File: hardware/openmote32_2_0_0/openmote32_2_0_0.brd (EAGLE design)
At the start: 24.1 x 32.8 mm, 39 parts, among them J1 XBEE_1-10, J2 XBEE_11-20, J3 JTAG_CONNECTOR, U1 AT86RF231, X1 16MHz

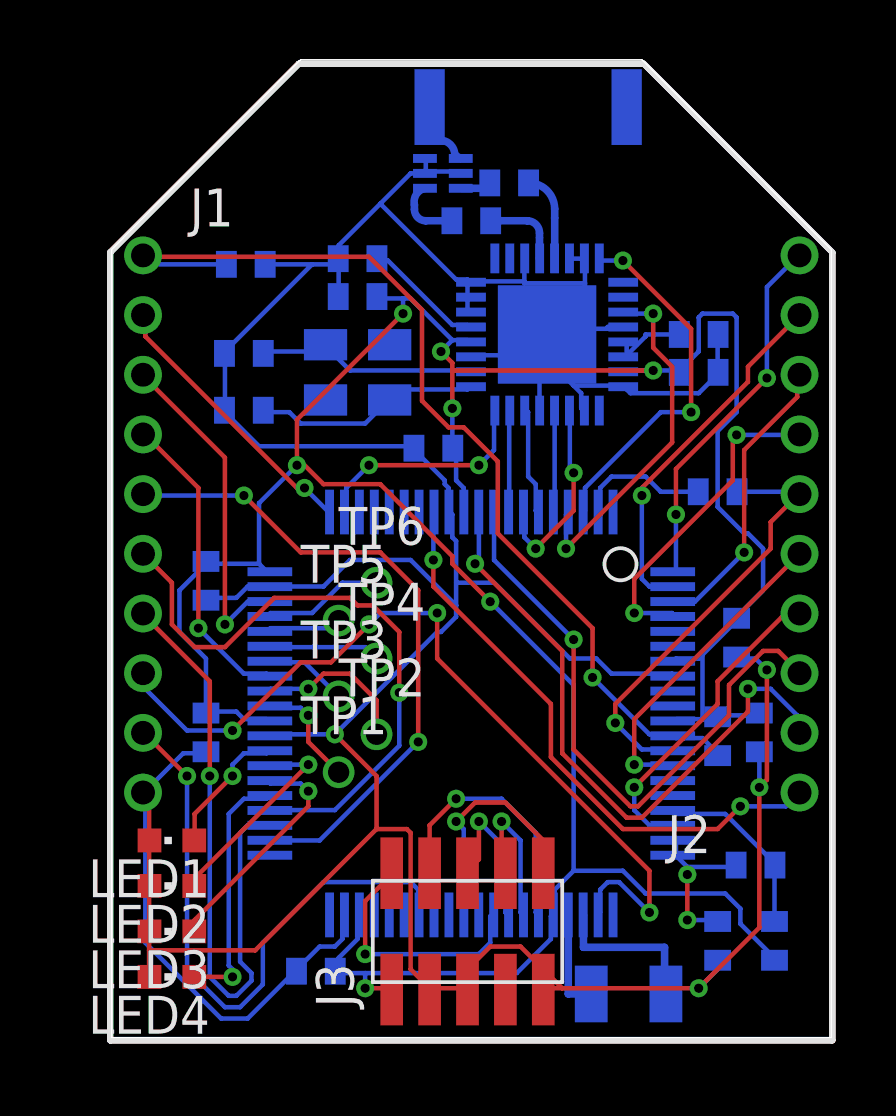
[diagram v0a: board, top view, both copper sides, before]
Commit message: Openmote v2 changes
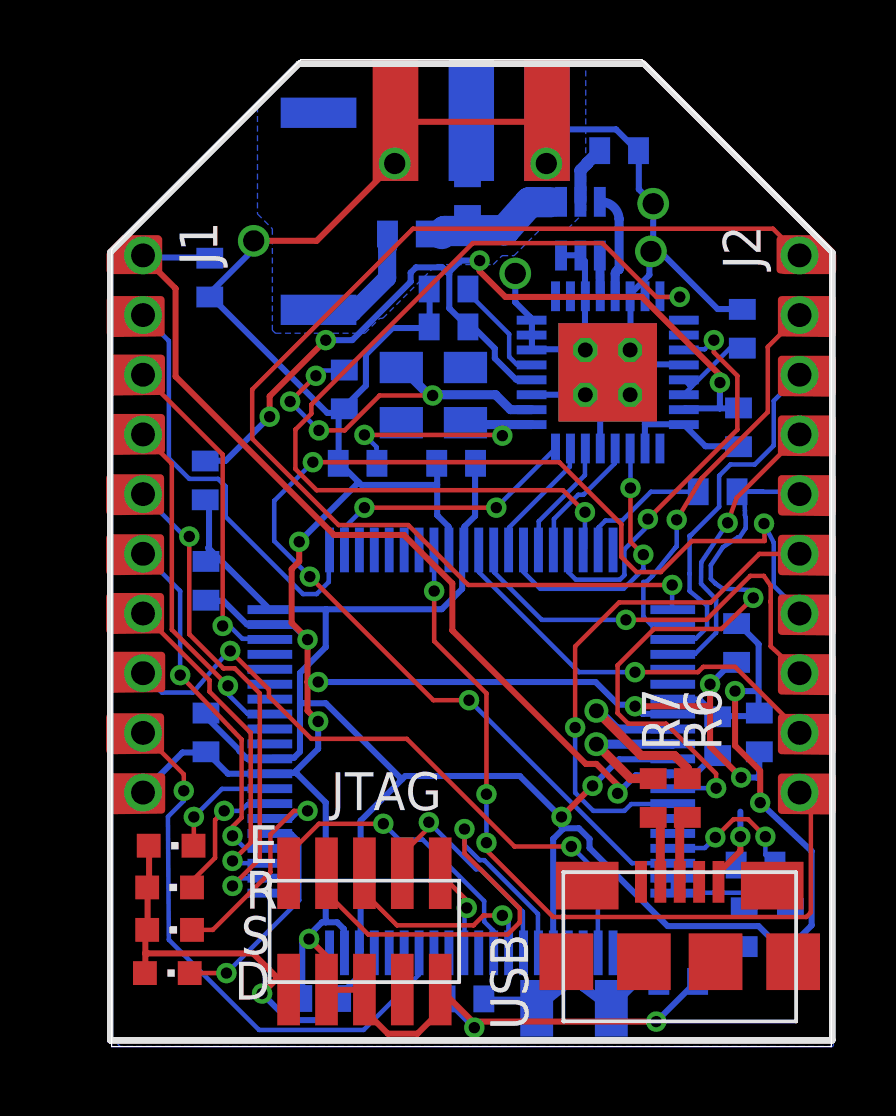
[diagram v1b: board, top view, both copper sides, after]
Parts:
- removed B1: BALUNG-TYPE, WSNlib:MURATA_LDB_BALUN
- removed C2: 22p, SparkFun:C0402
- removed TP1, TP2, TP3, TP4, TP5, TP6: TESTPOINTSMALLEST, WSNlib:TESTPOINT
- added C17, C18: 8p DNP, SparkFun:C0402
- added R3: 0R DNP, rcl:R0402
- added R4, R5: 0R, rcl:R0402
- added R6, R7: 33, rcl:R0402
- added TP10, TP11, TP12, TP7, TP8, TP9: TESTPOINTSMALLEST, WSNlib:TESTPOINT
- added U$1: DNP, WSNlib:CONREVSMA003.031
- added U$2: USB_CONNECTOR, WSNlib:MICROUSB_10118192
- added U3: 2450FB15L0001, WSNlib:2450FB15L0001
- J1: value XBEE_1-10 -> XBEE_1-10SMD; device WSNlib:XBEE_1-10 -> WSNlib:XBEE_1-10+SMD
- J2: value XBEE_11-20 -> XBEE_11-20SMD; device WSNlib:XBEE_11-20 -> WSNlib:XBEE_11-20+SMD
- R2: value 0R -> 0R DNP
- moved A1 7.84 mm to (6.95, 27.7), turned to 90 degrees
- moved C1 5.48 mm to (17.0, 29.7)
- moved C4 4.20 mm to (8.26, 19.2)
- moved C3 3.58 mm to (7.81, 21.7), turned to 90 degrees
- moved J3 3.45 mm to (8.48, 3.56)
- moved C8 3.21 mm to (11.3, 25.1)
- moved C6 3.21 mm to (11.3, 23.8)
- moved X1 2.65 mm to (10.8, 21.5)
- moved U1 2.40 mm to (16.6, 22.3)
- moved C5 2.27 mm to (21.0, 20.4), turned to 90 degrees
- moved X2 1.89 mm to (15.5, 0.98)
- moved C7 1.47 mm to (21.1, 23.7), turned to 90 degrees
- moved C9 1.29 mm to (3.30, 25.5), turned to 90 degrees
- moved U2 1.27 mm to (12.1, 9.59)
- moved L1 1.00 mm to (21.2, 3.70)
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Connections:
- new net N$12: A1.CON, R4.1
- new net N$15: R3.1, U$1.CON
- new net N$17: C5.2, C6.2, R5.2, U1.15, U1.28
- new net N$18: R7.2, U$2.2
- net 3.3V: now also LED1.A, LED2.A, LED3.A, LED4.A, R5.1; no longer C5.2, C6.2, U1.15, U1.28
- net DBG_FRAME: no longer TP1.P$1
- net DBG_FSM: no longer TP4.P$1
- net DBG_ISR: no longer TP6.P$1
- net DBG_RADIO: no longer TP3.P$1
- net DBG_SLOT: no longer TP2.P$1
- net DBG_TASK: no longer TP5.P$1
- net GND: now also C1.1, C17.1, C18.1, TP10.P$1, TP11.P$1, TP12.P$1, TP7.P$1, TP8.P$1, TP9.P$1, U$1.GND_1, U$1.GND_2, U$1.GND_3, U$1.GND_4, U$2.5, U1.P$1, U1.P$2, U1.P$3, U1.P$4, U1.PAD1, U3.5, U3.6; no longer B1.2, B1.5, B1.6, LED1.C, LED2.C, LED3.C, LED4.C
- net K20_USBDM: now also R7.1
- net K20_USBDP: now also R6.1
- net LED1: now also LED1.C; no longer LED1.A
- net LED2: now also LED2.C; no longer LED2.A
- net LED3: now also LED3.C; no longer LED3.A
- net LED4: now also LED4.C; no longer LED4.A
- net N$1: now also U1.4, U3.4; no longer B1.3, C2.2
- net N$11: now also C17.2
- net N$2: now also U1.5, U3.3; no longer B1.4, C1.2
- net N$3: now also R3.2, R4.2, U3.1; no longer A1.CON, B1.1
- net N$4: now also C1.2, U3.2; no longer C2.1, U1.5
- net N$5: now also R6.2, U$2.3; no longer C1.1, U1.4
- net N$8: now also C18.2
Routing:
- net XB_VREF: track 10.7 -> 42.8 mm, vias 1 -> 4
- net N$17: track 0.00 -> 30.7 mm, vias 0 -> 4
- net XB_AD0: track 12.4 -> 39.5 mm, vias 2 -> 1
- net RF231_#RST: track 12.3 -> 30.0 mm
- net 3.3V: track 104.3 -> 94.0 mm, vias 7 -> 5
- net XB_DIO11: track 21.2 -> 11.3 mm
- net XB_RSSI: track 20.9 -> 12.3 mm, vias 1 -> 2
- net JTAG_TCLK: track 8.79 -> 17.0 mm
- net XB_DIO7: track 21.3 -> 13.9 mm, vias 2 -> 1
- net XB_AD4: track 19.7 -> 26.8 mm, vias 2 -> 3
- net K20_USBDP: track 0.00 -> 7.00 mm, vias 0 -> 1
- net XB_AD6: track 14.7 -> 21.4 mm, vias 1 -> 2
- net XB_AD5: track 10.7 -> 17.3 mm
- net XB_EXTRA: track 28.6 -> 22.1 mm, vias 4 -> 2
- net XB_ON: track 20.5 -> 14.8 mm
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- added copper zone on layer 16, net GND
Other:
- board size 24.1 x 32.8 mm -> 24.1 x 33.1 mm
- board text added: "D"
- board text added: "E"
- board text added: "JTAG"
- board text added: "R"
- board text added: "S"
- board text added: "USB"
